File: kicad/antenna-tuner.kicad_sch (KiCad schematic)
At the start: 0 parts

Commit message: Partial kicad schematic
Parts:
- added A1: Pololu_Breakout_A4988, Module:Pololu_Breakout-16_15.2x20.3mm, symbol Driver_Motor:Pololu_Breakout_A4988
- added C1: 100uF, symbol Device:C_Polarized
- added M1: Stepper_Motor_bipolar, symbol Motor:Stepper_Motor_bipolar
- added R1, R2, R3: 100k, symbol Device:R
- added SW1: RIGHT_FINE, symbol Switch:SW_SPST
- added SW2: RIGHT_COARSE, symbol Switch:SW_SPST
- added SW3: LEFT_COARSE, symbol Switch:SW_SPST
- added SW4: LEFT_FINE, symbol Switch:SW_SPST
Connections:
- new net: A1.13 (~{RESET}), R3.2
- new net: A1.14 (~{SLEEP}), R2.2
- new net: A1.3 (1B), M1.2 (-)
- new net: A1.4 (1A), M1.1
- new net: A1.5 (2A), M1.3
- new net: A1.6 (2B), M1.4
- new net: A1.9 (~{ENABLE}), R1.2
- new net 12V: A1.8 (VMOT), C1.1
- new net GND: A1.1 (GND), C1.2, R1.1, R2.1, R3.1, SW1.1 (A), SW2.1 (A), SW3.1 (A), SW4.1 (A)
- new net TINY_3 (PD5): A1.15 (STEP)
- new net TINY_4 (PD6): A1.16 (DIR)
- new net TINY_5V: A1.2 (VDD)
- new net TINY_A2 (PC2): SW1.2 (B)
- new net TINY_A4 (PC3): SW2.2 (B)
- new net TINY_A4 (PC4): SW3.2 (B)
- new net TINY_A5 (PC5): SW4.2 (B)
- no-connect marks 0 -> 1
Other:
- note added: "Built-in pull-up resistors"
- note added: "Step-down module"

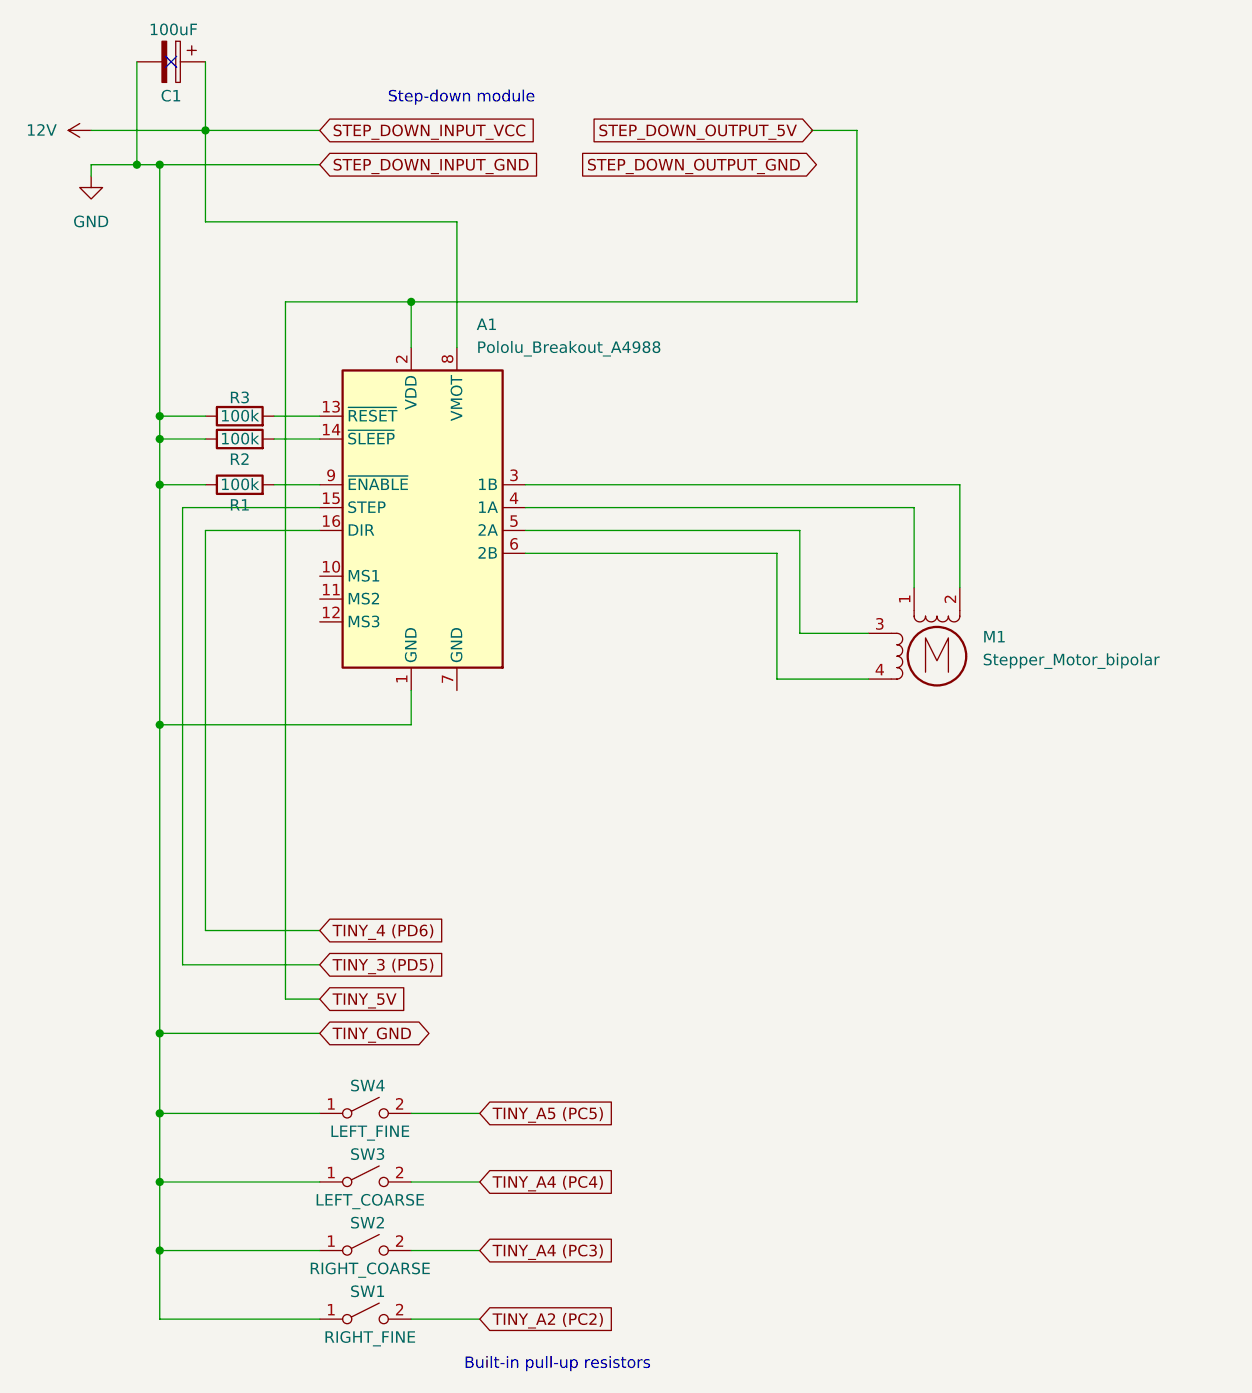
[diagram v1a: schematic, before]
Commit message: Updated schematic
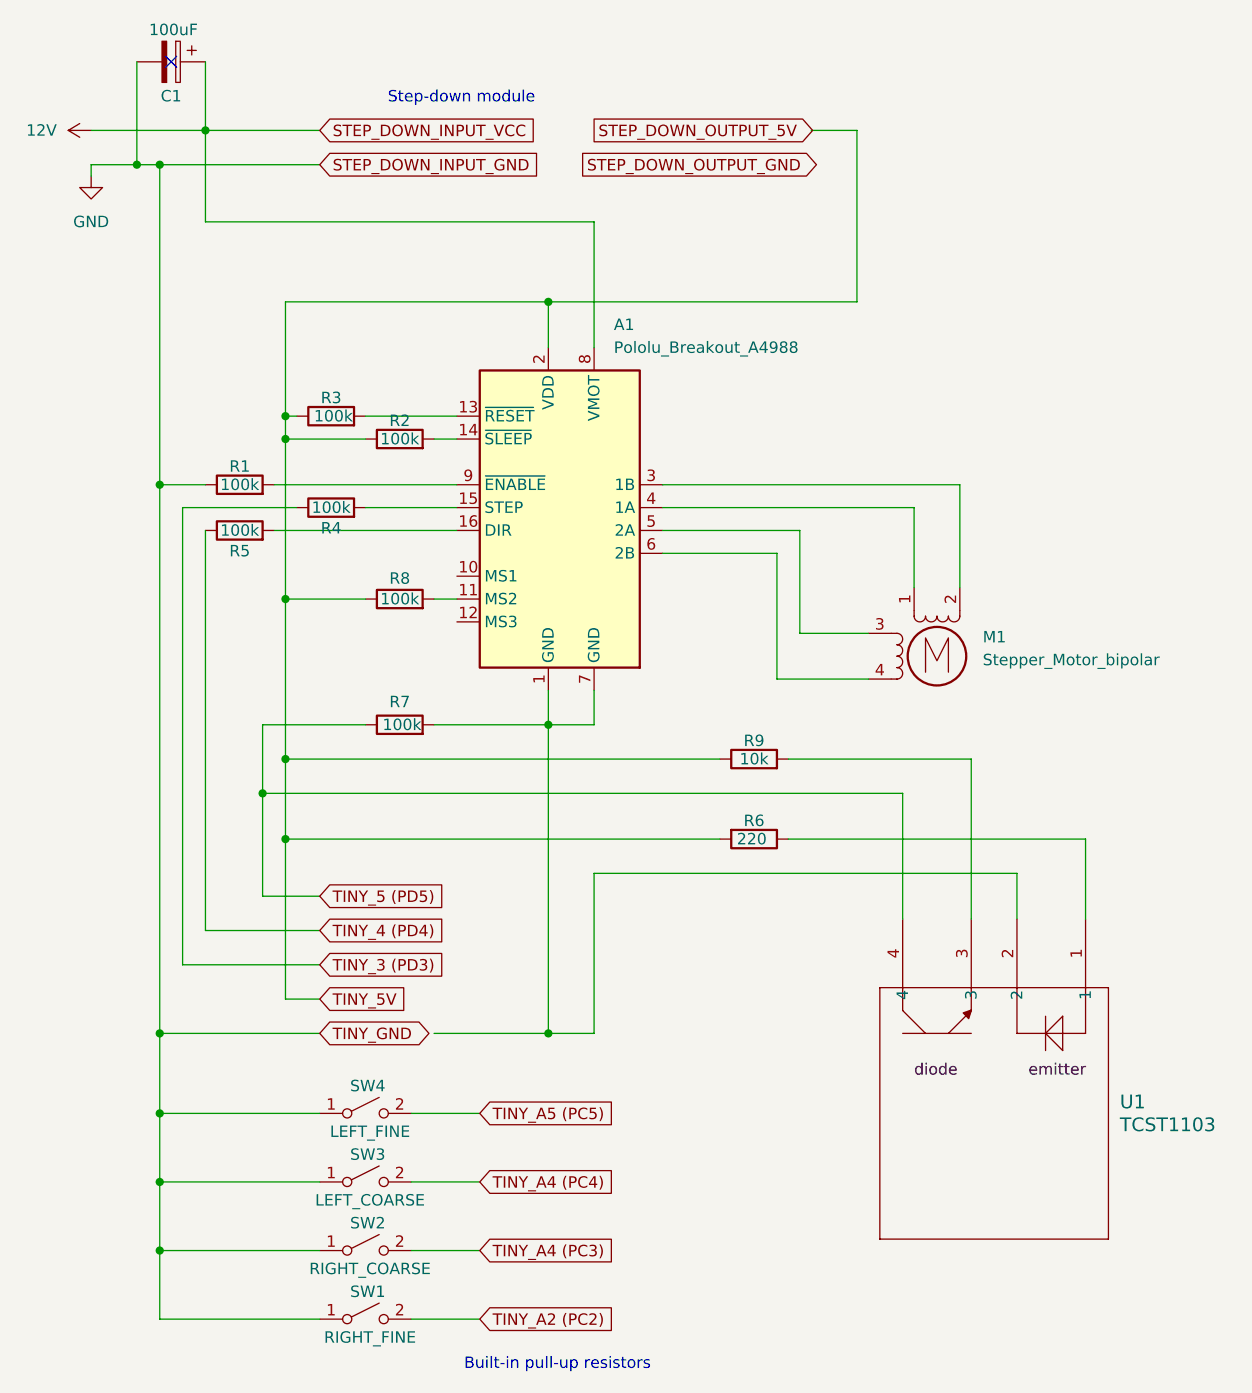
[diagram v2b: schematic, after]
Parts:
- added R4, R5, R7, R8: 100k, symbol Device:R
- added R6: 220, symbol Device:R
- added R9: 10k, symbol Device:R
- added U1: TCST1103, TCRT1010_VIS, symbol 2024-12-14_18-26-05:TCST1103
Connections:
- net GND: no longer A1.1 (GND), R2.1, R3.1
- net TINY_5V: now also R2.1, R3.1, R6.2, R8.1, R9.1
- net at A1.11 (MS2): now also R8.2
- net at A1.7 (GND): now also A1.1 (GND), R7.2, U1.2
- net TINY_3 (PD5): no longer names the net of A1.15 (STEP)
- net TINY_3 (PD5): now also R4.2
- net TINY_4 (PD6): no longer names the net of A1.16 (DIR)
- net TINY_4 (PD6): now also R5.2
- new net: R6.1, U1.1
- new net: R9.2, U1.3
- new net TINY_3 (PD3): R4.1
- new net TINY_4 (PD4): R5.1
- new net TINY_5 (PD5): R7.1, U1.4
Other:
- moved on the sheet: A1, R2, R3
